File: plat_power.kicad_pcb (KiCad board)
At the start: 2 copper layers, 147.3 x 123.8 mm, 167 parts, among them Con3 DG125-5.0-02P-14-00A(H), J1 Conn_01x18_Pin, J2 Conn_01x18_Pin, J3 Conn_01x06_Pin, U1 LD39050PU33R, U10 DRV8873SPWPRQ1, U11 DRV8873SPWPRQ1, U12 REF5025AD, U13 ISO7762FDBQ, U14 ISO7762FDBQ, U15 ISO7762FDBQ, U16 TLV9061xDBV, U17 ISO7762FDBQ, U18 ISO7762FDBQ, U19 ISO7762FDBQ, U2 TPS5450, U20 ISO7762FDBQ, U3 ISO1540, U4 TPS5450, U5 TPS5450, U6 DRV8873SPWPRQ1, U7 DRV8873SPWPRQ1, U8 DRV8873SPWPRQ1, U9 DRV8873SPWPRQ1, con4 KF202

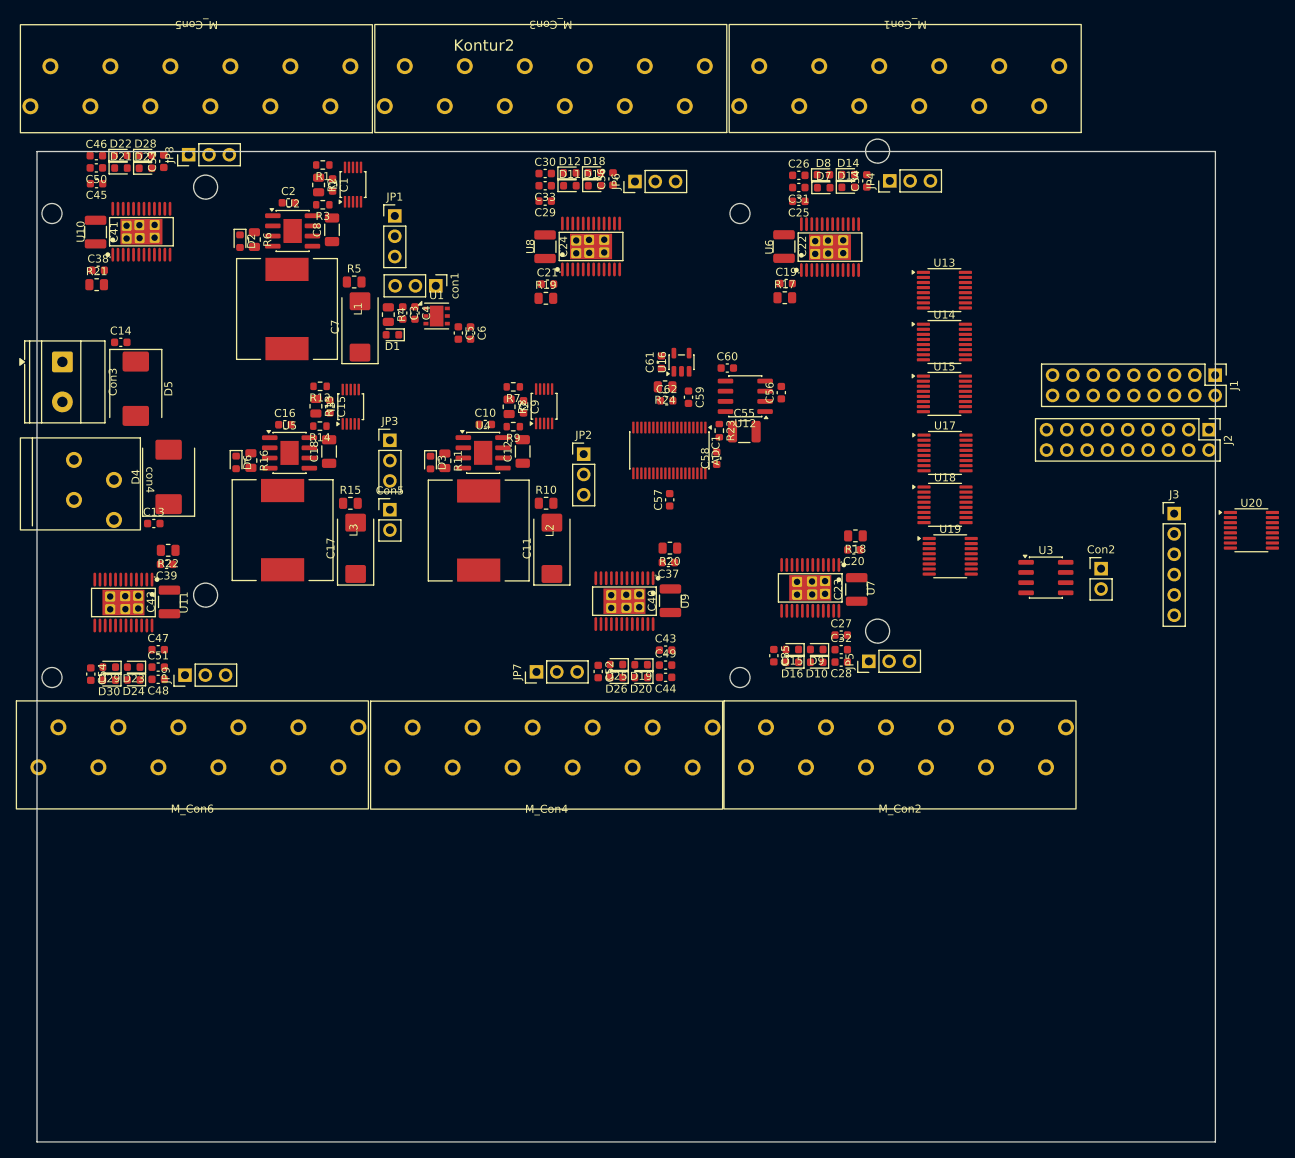
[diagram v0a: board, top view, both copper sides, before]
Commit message: tray
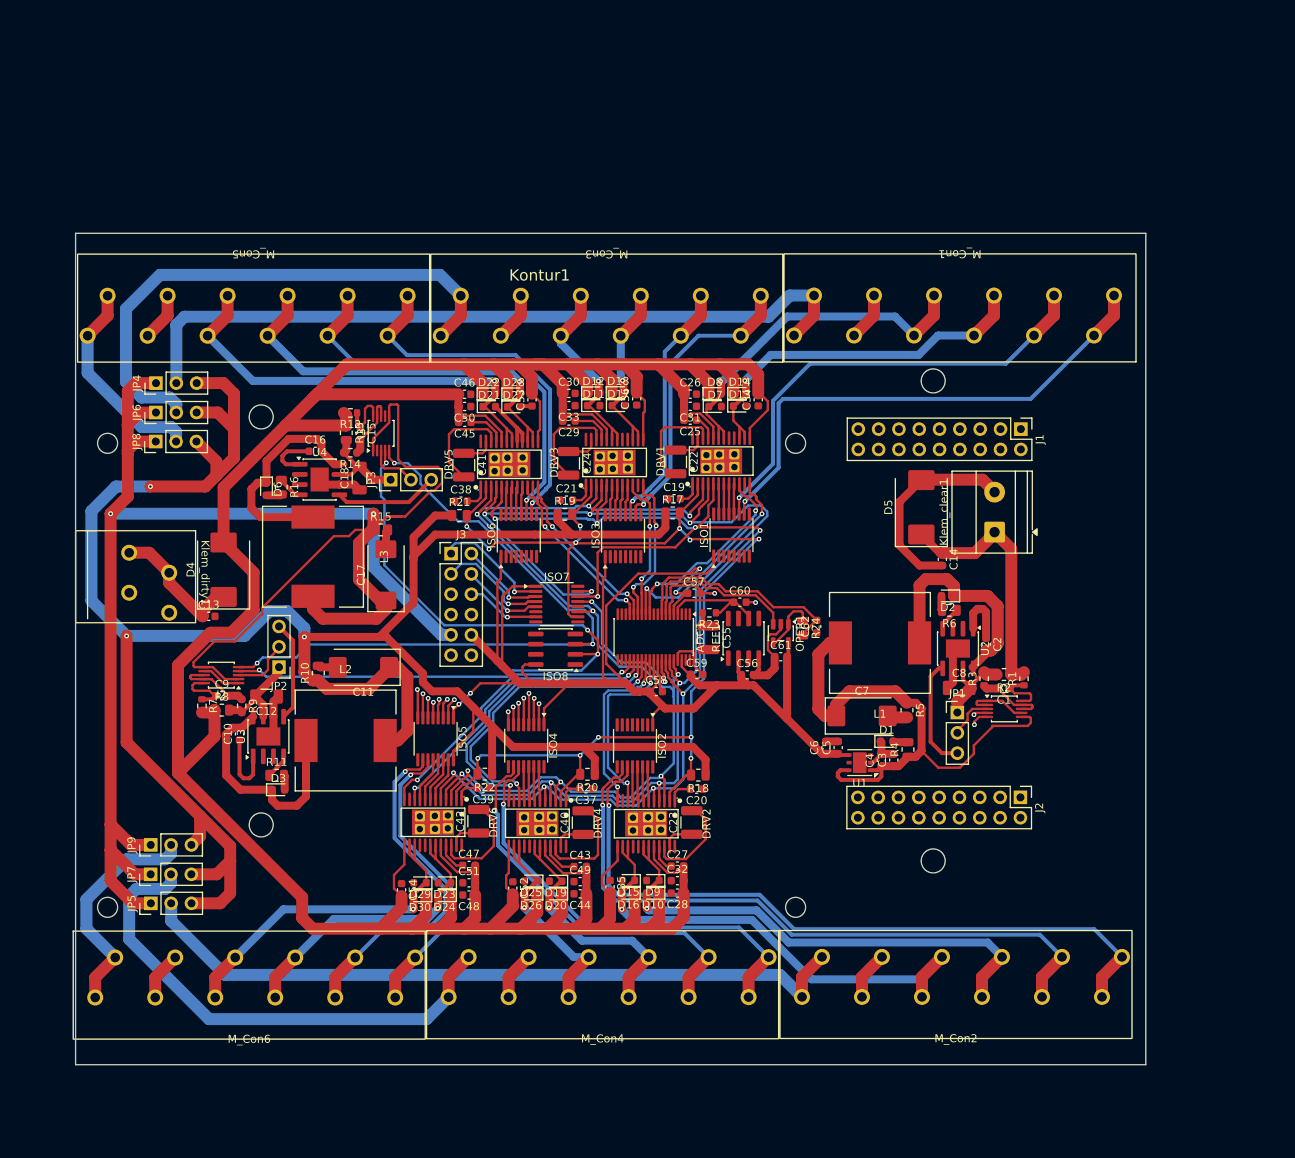
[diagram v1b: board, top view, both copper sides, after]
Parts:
- removed Con2, Con5: ~, Connector_PinHeader_2.54mm:PinHeader_1x02_P2.54mm_Vertical
- removed Con3: DG125-5.0-02P-14-00A(H), TerminalBlock_Phoenix:TerminalBlock_Phoenix_MKDS-1,5-2_1x02_P5.00mm_Horizontal
- removed Kontur2: ~, Library_footprints:JetBot_AI_Kit_3x18650_Hole_Pattern
- removed U10, U11, U6, U7, U8, U9: DRV8873SPWPRQ1, Library_footprints:C2150678_HTSSOP-24_L7_8-W4_4-P0_65-LS6_4-TL-EP
- removed U12: REF5025AD, Package_SO:SOIC-8_3.9x4.9mm_P1.27mm
- removed U13, U14, U15, U17, U18, U19, U20: ISO7762FDBQ, Package_SO:SSOP-16_3.9x4.9mm_P0.635mm
- removed U16: TLV9061xDBV, Package_TO_SOT_SMD:SOT-23-5
- removed U5: TPS5450, Package_SO:SOIC-8-1EP_3.9x4.9mm_P1.27mm_EP2.29x3mm
- removed con1: ~, Connector_PinHeader_2.54mm:PinHeader_1x03_P2.54mm_Vertical
- removed con4: KF202, Library_footprints:con_klemnic
- added DRV1: DRV8873SPWPRQ1, Library_footprints:C2150678_HTSSOP-24_L7_8-W4_4-P0_65-LS6_4-TL-EP, F.Cu at (166.7, 77.6)
- added DRV2: DRV8873SPWPRQ1, Library_footprints:C2150678_HTSSOP-24_L7_8-W4_4-P0_65-LS6_4-TL-EP, F.Cu at (157.3, 122.9)
- added DRV3: DRV8873SPWPRQ1, Library_footprints:C2150678_HTSSOP-24_L7_8-W4_4-P0_65-LS6_4-TL-EP, F.Cu at (153.4, 77.8)
- added DRV4: DRV8873SPWPRQ1, Library_footprints:C2150678_HTSSOP-24_L7_8-W4_4-P0_65-LS6_4-TL-EP, F.Cu at (143.8, 122.9)
- added DRV5: DRV8873SPWPRQ1, Library_footprints:C2150678_HTSSOP-24_L7_8-W4_4-P0_65-LS6_4-TL-EP, F.Cu at (140.2, 78.0)
- added DRV6: DRV8873SPWPRQ1, Library_footprints:C2150678_HTSSOP-24_L7_8-W4_4-P0_65-LS6_4-TL-EP, F.Cu at (130.7, 122.8)
- added ISO1: ISO7762FDBQ, Package_SO:SSOP-16_3.9x4.9mm_P0.635mm, F.Cu at (168.0, 86.8)
- added ISO2: ISO7762FDBQ, Package_SO:SSOP-16_3.9x4.9mm_P0.635mm, F.Cu at (155.9, 113.2)
- added ISO3: ISO7762FDBQ, Package_SO:SSOP-16_3.9x4.9mm_P0.635mm, F.Cu at (154.5, 86.9)
- added ISO4: ISO7762FDBQ, Package_SO:SSOP-16_3.9x4.9mm_P0.635mm, F.Cu at (142.4, 113.2)
- added ISO5: ISO7762FDBQ, Package_SO:SSOP-16_3.9x4.9mm_P0.635mm, F.Cu at (131.0, 112.3)
- added ISO6: ISO7762FDBQ, Package_SO:SSOP-16_3.9x4.9mm_P0.635mm, F.Cu at (141.4, 86.9)
- added ISO7: ISO7762FDBQ, Package_SO:SSOP-16_3.9x4.9mm_P0.635mm, F.Cu at (146.2, 95.5)
- added ISO8: ISO1540, Package_SO:SOIC-8_3.9x4.9mm_P1.27mm, F.Cu at (146.0, 101.1)
- added Klem_clear1: DG125-5.0-02P-14-00A(H), TerminalBlock_Phoenix:TerminalBlock_Phoenix_MKDS-1,5-2_1x02_P5.00mm_Horizontal, F.Cu at (200.9, 86.5)
- added Klem_dirty1: KF202, Library_footprints:con_klemnic, F.Cu at (86.0, 86.3)
- added Kontur1: ~, Library_footprints:JetBot_AI_Kit_3x18650_Hole_Pattern, F.Cu at (86.0, 58.4)
- added OPER1: TLV9061xDBV, Package_TO_SOT_SMD:SOT-23-5, F.Cu at (174.2, 99.1)
- added REF1: REF5025AD, Package_SO:SOIC-8_3.9x4.9mm_P1.27mm, F.Cu at (169.5, 99.8)
- J3: value Conn_01x06_Pin -> Conn_01x12_Pin; footprint Connector_PinHeader_2.54mm:PinHeader_1x06_P2.54mm_Vertical -> Connector_PinHeader_2.54mm:PinHeader_2x06_P2.54mm_Vertical
- U3: value ISO1540 -> TPS5450; footprint Package_SO:SOIC-8_3.9x4.9mm_P1.27mm -> Package_SO:SOIC-8-1EP_3.9x4.9mm_P1.27mm_EP2.29x3mm
- moved R1 108.7 mm to (204.6, 104.8), turned to 90 degrees
- moved C14 106.2 mm to (194.4, 89.9), turned to -90 degrees
- moved R2 105.3 mm to (202.1, 104.3), turned to 180 degrees
- moved C1 104.9 mm to (202.1, 106.0), turned to 180 degrees
- moved I1 104.5 mm to (202.1, 108.6), turned to 0 degrees
- moved C2 103.2 mm to (199.8, 100.5), turned to -90 degrees
- moved R3 101.7 mm to (199.6, 104.8), turned to 90 degrees
- moved D5 99.3 mm to (191.7, 83.4), turned to 90 degrees
- moved U3 99.2 mm to (110.1, 112.0), turned to 90 degrees
- moved D2 99.0 mm to (195.0, 94.5), turned to 180 degrees
- moved R6 98.5 mm to (195.2, 96.2), turned to 180 degrees
- moved U2 98.2 mm to (196.3, 101.0), turned to -90 degrees
- moved C8 97.1 mm to (196.5, 106.0), turned to 0 degrees
- moved JP4 95.1 mm to (96.1, 67.8)
- moved JP5 94.7 mm to (95.4, 132.9)
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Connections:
- ADC1 pad 13: IPROPI1_2 -> IPROPI1_3
- ADC1 pad 14: IPROPI2_2 -> IPROPI2_3
- ADC1 pad 15: IPROPI1_3 -> IPROPI2_5
- ADC1 pad 16: IPROPI2_3 -> IPROPI1_5
- ADC1 pad 25: IPROPI2_5 -> IPROPI2_4
- ADC1 pad 26: IPROPI1_5 -> IPROPI1_4
- ADC1 pad 27: IPROPI2_4 -> IPROPI2_2
- ADC1 pad 28: IPROPI1_4 -> IPROPI1_2
- C10 pad 1: Net-(U4-BOOT) -> Net-(U3-BOOT)
- C16 pad 1: Net-(U5-BOOT) -> Net-(U4-BOOT)
- J1 pad 10: DISABLE_mk_2 -> DISABLE_mk_3
- J1 pad 11: ENC_A_M2_mk -> ENC_A_M3_mk
- J1 pad 12: ENC_B_M2_mk -> ENC_B_M3_mk
- J1 pad 13: nSCS_mk_3 -> nSCS_mk_5
- J1 pad 14: EN/IN1_mk_3 -> EN/IN1_mk_5
- J1 pad 15: PH/IN2_mk_3 -> PH/IN2_mk_5
- J1 pad 16: DISABLE_mk_3 -> DISABLE_mk_5
- J1 pad 17: ENC_A_M3_mk -> ENC_A_M5_mk
- J1 pad 18: ENC_B_M3_mk -> ENC_B_M5_mk
- J1 pad 7: nSCS_mk_2 -> nSCS_mk_3
- J1 pad 8: EN/IN1_mk_2 -> EN/IN1_mk_3
- J1 pad 9: PH/IN2_mk_2 -> PH/IN2_mk_3
- J2 pad 1: nSCS_mk_4 -> nSCS_mk_2
- J2 pad 10: DISABLE_mk_5 -> DISABLE_mk_4
- J2 pad 11: ENC_A_M5_mk -> ENC_A_M4_mk
- J2 pad 12: ENC_B_M5_mk -> ENC_B_M4_mk
- J2 pad 2: EN/IN1_mk_4 -> EN/IN1_mk_2
- J2 pad 3: PH/IN2_mk_4 -> PH/IN2_mk_2
- J2 pad 4: DISABLE_mk_4 -> DISABLE_mk_2
- J2 pad 5: ENC_A_M4_mk -> ENC_A_M2_mk
- J2 pad 6: ENC_B_M4_mk -> ENC_B_M2_mk
- J2 pad 7: nSCS_mk_5 -> nSCS_mk_4
- J2 pad 8: EN/IN1_mk_5 -> EN/IN1_mk_4
- J2 pad 9: PH/IN2_mk_5 -> PH/IN2_mk_4
- J3 pad 5: unconnected-(J3-Pin_5-Pad5) -> Net-(ISO8-SDA2)
- M_Con1 pad 1: CONN_2_M1 -> Net-(JP4-C)
- M_Con1 pad 2: CONN_1_M1 -> GND
- M_Con1 pad 3: Net-(JP4-C) -> CONN_1_M1
- M_Con1 pad 4: ENC_B_M1 -> CONN_2_M1
- M_Con1 pad 6: GND -> ENC_B_M1
- M_Con2 pad 1: CONN_2_M2 -> ENC_A_M2
- M_Con2 pad 2: CONN_1_M2 -> ENC_B_M2
- M_Con2 pad 3: Net-(JP5-C) -> CONN_1_M2
- M_Con2 pad 4: ENC_B_M2 -> CONN_2_M2
- M_Con2 pad 5: ENC_A_M2 -> GND
- M_Con2 pad 6: GND -> Net-(JP5-C)
- M_Con3 pad 1: CONN_2_M3 -> Net-(JP6-C)
- M_Con3 pad 2: CONN_1_M3 -> GND
- M_Con3 pad 3: Net-(JP6-C) -> CONN_1_M3
- M_Con3 pad 4: ENC_B_M3 -> CONN_2_M3
- M_Con3 pad 6: GND -> ENC_B_M3
- M_Con4 pad 1: CONN_2_M4 -> ENC_A_M4
- M_Con4 pad 2: CONN_1_M4 -> ENC_B_M4
- M_Con4 pad 3: Net-(JP7-C) -> CONN_1_M4
- M_Con4 pad 4: ENC_B_M4 -> CONN_2_M4
- M_Con4 pad 5: ENC_A_M4 -> GND
- M_Con4 pad 6: GND -> Net-(JP7-C)
- M_Con5 pad 1: CONN_2_M5 -> Net-(JP8-C)
- M_Con5 pad 2: CONN_1_M5 -> GND
- M_Con5 pad 3: Net-(JP8-C) -> CONN_1_M5
- M_Con5 pad 4: ENC_B_M5 -> CONN_2_M5
- M_Con5 pad 6: GND -> ENC_B_M5
- M_Con6 pad 1: CONN_2_M6 -> ENC_A_M6
- M_Con6 pad 2: CONN_1_M6 -> ENC_B_M6
- M_Con6 pad 3: Net-(JP9-C) -> CONN_1_M6
- M_Con6 pad 4: ENC_B_M6 -> CONN_2_M6
- M_Con6 pad 5: ENC_A_M6 -> GND
- M_Con6 pad 6: GND -> Net-(JP9-C)
- R11 pad 1: Net-(U4-VSENSE) -> Net-(U3-VSENSE)
- R16 pad 1: Net-(U5-VSENSE) -> Net-(U4-VSENSE)
- U3 pad 1: +3,3v -> Net-(U3-BOOT)
- U3 pad 2: SDA_INA -> unconnected-(U3-NC-Pad2)
- U3 pad 3: SCL_INA -> unconnected-(U3-NC-Pad3)
- U3 pad 4: GND -> Net-(U3-VSENSE)
- U3 pad 5: GND* -> ENA_U4
- U3 pad 6: Net-(U3-SCL2) -> GND
- U3 pad 7: Net-(U3-SDA2) -> Net-(JP2-A)
- U3 pad 8: +3,3v* -> Net-(D3-K)
- U4 pad 5: ENA_U4 -> ENA_U5
- U4 pad 7: Net-(JP2-A) -> Net-(JP3-A)
- U4 pad 8: Net-(D3-K) -> Net-(D6-K)
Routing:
- net +14.4v: track 0.00 -> 444.8 mm
- net +3,3v: track 0.00 -> 307.8 mm, vias 0 -> 3
- net +5v: track 0.00 -> 243.5 mm, vias 0 -> 2
- net +3,3v*: track 0.00 -> 186.4 mm, vias 0 -> 4
- net SCLK_ISO: track 0.00 -> 153.1 mm, vias 0 -> 9
- net SDI_ISO: track 0.00 -> 152.3 mm, vias 0 -> 8
- net nFault_ISO: track 0.00 -> 150.6 mm, vias 0 -> 12
- net SDO_ISO: track 0.00 -> 132.3 mm, vias 0 -> 8
- net SDA_INA: track 0.00 -> 98.4 mm, vias 0 -> 5
- net Net-(JP4-C): track 0.00 -> 94.5 mm
- net Net-(JP5-C): track 0.00 -> 91.0 mm
- net ENC_A_M2: track 0.00 -> 90.3 mm, vias 0 -> 1
- net GND*: track 0.00 -> 88.7 mm, vias 0 -> 4
- net SCL_INA: track 0.00 -> 88.4 mm, vias 0 -> 4
- net ENC_B_M2: track 0.00 -> 83.6 mm, vias 0 -> 1
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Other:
- board size 147.3 x 123.8 mm -> 133.8 x 103.9 mm
